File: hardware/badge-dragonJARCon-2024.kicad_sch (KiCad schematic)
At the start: 32 parts, among them J1 UART, J2 Battery, J3 OLED, J5 Shitty addon, P1 USB_C_Plug_USB2.0, Q1 DMG3415U-7, SW1 ON, SW2 RESET, SW3 BOOT, SW4 PB4, SW5 PB3, SW6 PB1, SW7 PB2, U1 ESP32-C6-WROOM-1U-N4, U2 AP2112K-3.3

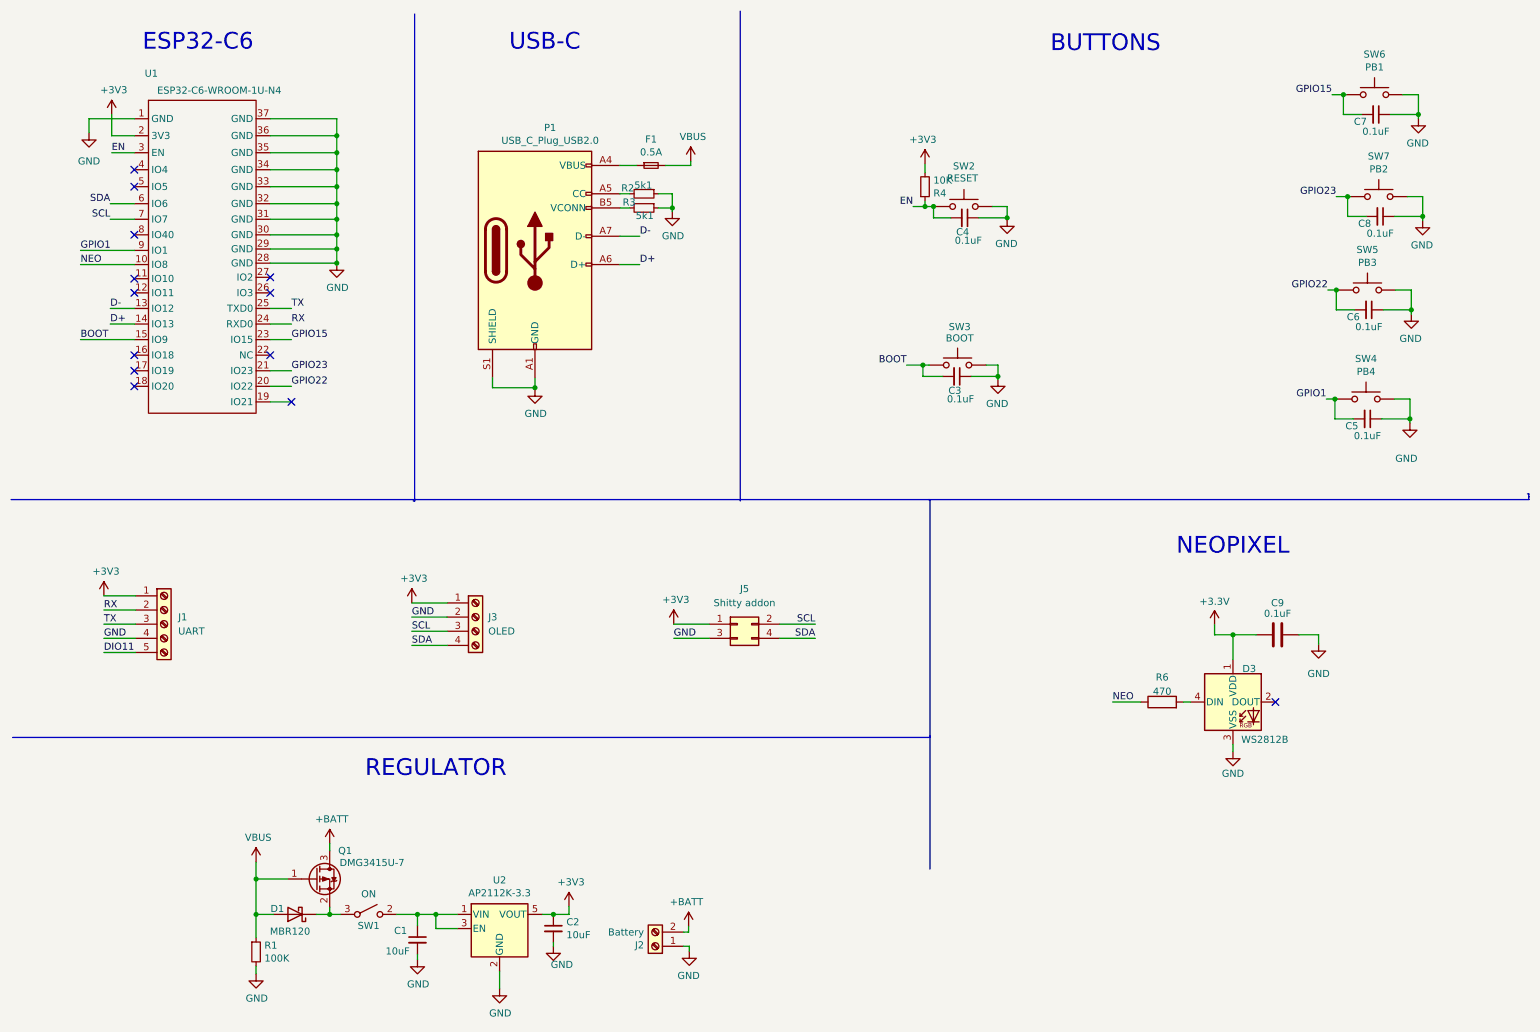
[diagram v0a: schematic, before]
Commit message: feat(Hw): Init floorplan
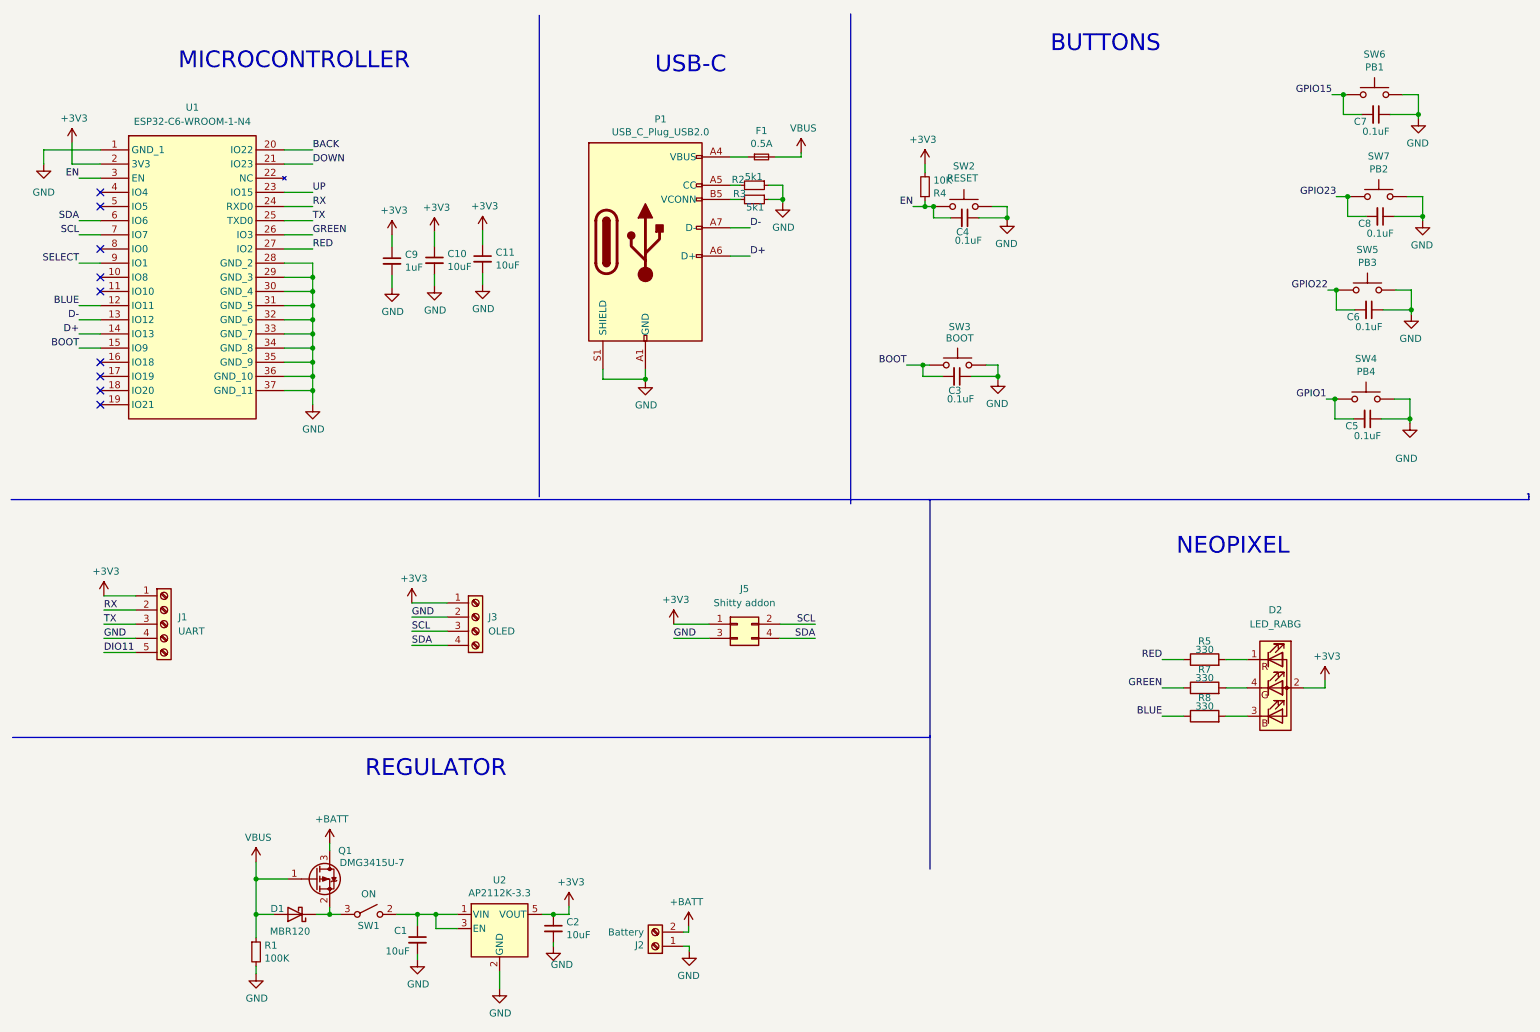
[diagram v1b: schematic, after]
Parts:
- removed C9: 0.1uF, Capacitor_SMD:C_0603_1608Metric, symbol Device:C
- removed D3: WS2812B, Ekoparty:LED_SK6812MINI_PLCC4_3.5x3.5mm_P1.75mm, symbol LED:WS2812B
- removed R6: 470, Resistor_SMD:R_0603_1608Metric, symbol Device:R
- removed U1: ESP32-C6-WROOM-1U-N4, Footprint:MOD28_ESP32-C6-WROOM-1U_EXP, symbol Minino:ESP32-C6-WROOM-1U-N8
- added C10, C11: 10uF, Capacitor_SMD:C_0603_1608Metric, symbol Device:C_Small
- added C9: 1uF, Capacitor_SMD:C_0603_1608Metric, symbol Device:C_Small
- added D2: LED_RABG, Footprints:AAA3528SURKCGKC09, symbol Device:LED_RABG
- added R5, R7, R8: 330, Resistor_SMD:R_0603_1608Metric, symbol Device:R
- added U1: ESP32-C6-WROOM-1-N4, Footprints:ESP32C6WROOM1N4, symbol ESP32-C6-WROOM-1-N4:ESP32-C6-WROOM-1-N4
- J2: footprint Footprint:BAT-TH_BH-AAA-A1AJ024 -> Footprints:BAT-TH_BH-AAA-A1AJ024
- J3: footprint Connector_PinHeader_2.54mm:PinHeader_1x04_P2.54mm_Vertical -> Footprints:Display OLED 128 x32
- J5: footprint (none) -> Connector_PinHeader_2.54mm:PinHeader_2x02_P2.54mm_Vertical
- P1: footprint Footprint:C393939 -> Footprints:C393939
- SW1: footprint Footprint:JS102011SAQN -> Footprints:JS102011SAQN
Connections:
- net +3V3: now also C10.1, C11.1, C9.1, D2.2 (A), U1.2 (3V3)
- net BOOT: now also U1.15 (IO9)
- net D+: now also U1.14 (IO13)
- net D-: now also U1.13 (IO12)
- net EN: now also U1.3 (EN)
- net GND: now also C10.2, C11.2, C9.2, U1.1 (GND_1), U1.28 (GND_2), U1.29 (GND_3), U1.30 (GND_4), U1.31 (GND_5), U1.32 (GND_6), U1.33 (GND_7), U1.34 (GND_8), U1.35 (GND_9), U1.36 (GND_10), U1.37 (GND_11)
- net RX: now also U1.24 (RXD0)
- net SCL: now also U1.7 (IO7)
- net SDA: now also U1.6 (IO6)
- net TX: now also U1.25 (TXD0)
- new net: D2.1 (RK), R5.2
- new net: D2.3 (BK), R8.2
- new net: D2.4 (GK), R7.2
- new net BACK: U1.20 (IO22)
- new net BLUE: R8.1, U1.12 (IO11)
- new net DOWN: U1.21 (IO23)
- new net GREEN: R7.1, U1.26 (IO3)
- new net RED: R5.1, U1.27 (IO2)
- new net SELECT: U1.9 (IO1)
- new net UP: U1.23 (IO15)
- no-connect marks 13 -> 9
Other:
- note added: "MICROCONTROLLER"
- note removed: "ESP32-C6"
- moved on the sheet: F1, P1, R2, R3
